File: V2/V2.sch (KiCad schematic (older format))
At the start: 183 parts, among them U1 Elite-C

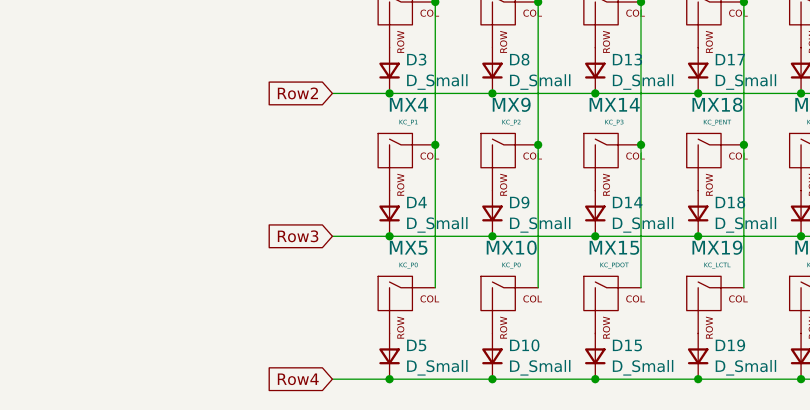
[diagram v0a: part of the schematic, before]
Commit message: Updated schematic and pcb design
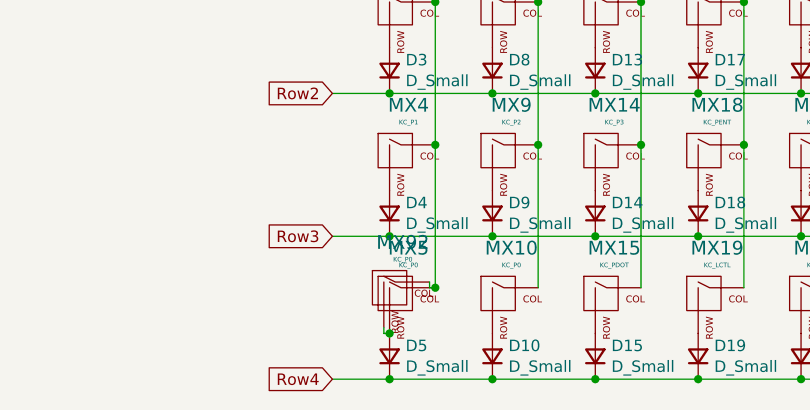
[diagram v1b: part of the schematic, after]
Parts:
- added MX92: KC_P0, MX_Alps_Hybrid:MXOnly-2U-Hotswap-ReversedStabilizers, symbol MX_Alps_Hybrid:MX-NoLED
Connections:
- net Col0: now also MX92.1 (COL)
- net at D5.2 (A), MX5.2 (ROW): now also MX92.2 (ROW)
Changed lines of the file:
@@
 Wire Wire Line
 	9075 2900 9975 2900
+$Comp
+L MX_Alps_Hybrid:MX-NoLED MX92
+U 1 1 60EC3BEF
+P 3275 3775
+F 0 "MX92" H 3308 3998 60  0000 C CNN
+F 1 "KC_P0" H 3308 3924 20  0000 C CNN
+F 2 "MX_Alps_Hybrid:MXOnly-2U-Hotswap-ReversedStabilizers" H 2650 3750 60  0001 C CNN
+F 3 "" H 2650 3750 60  0001 C CNN
+	1    3275 3775
+	1    0    0    -1
+$EndComp
+Wire Wire Line
+	3425 3725 3425 3750
+Wire Wire Line
+	3425 3750 3450 3750
+Connection ~ 3450 3750
+Wire Wire Line
+	3225 3925 3225 3950
+Wire Wire Line
+	3225 3950 3250 3950
+Connection ~ 3250 3950
 $EndSCHEMATC

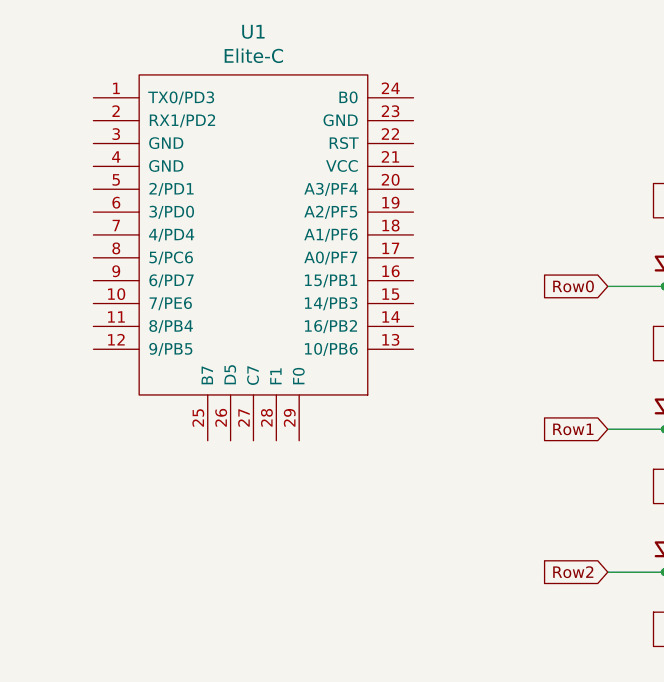
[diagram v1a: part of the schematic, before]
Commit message: Finished PCB
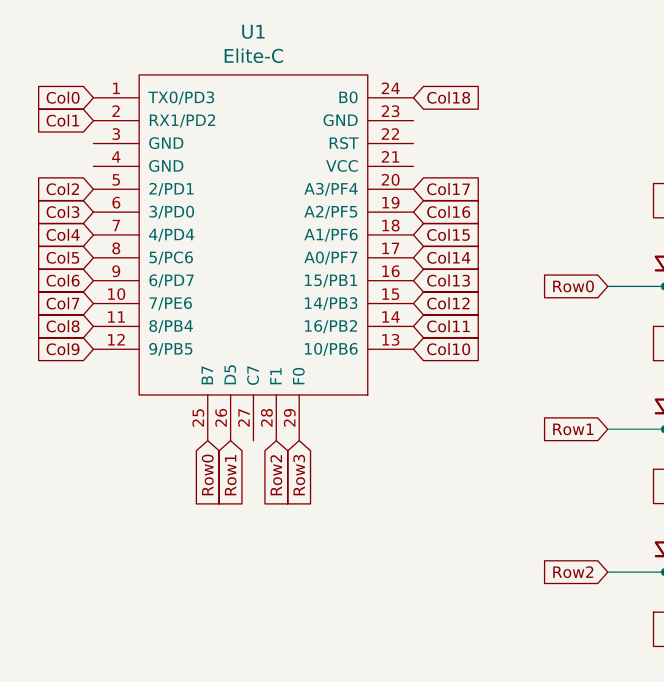
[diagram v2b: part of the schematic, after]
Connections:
- net Col0: now also U1.1 (TX0/PD3)
- net Col1: now also U1.2 (RX1/PD2)
- net Col10: now also U1.13 (10/PB6)
- net Col11: now also U1.14 (16/PB2)
- net Col12: now also U1.15 (14/PB3)
- net Col13: now also U1.16 (15/PB1)
- net Col14: now also U1.17 (A0/PF7)
- net Col15: now also U1.18 (A1/PF6)
- net Col16: now also U1.19 (A2/PF5)
- net Col17: now also U1.20 (A3/PF4)
- net Col18: now also U1.24 (B0)
- net Col2: now also U1.5 (2/PD1)
- net Col3: now also U1.6 (3/PD0)
- net Col4: now also U1.7 (4/PD4)
- net Col5: now also U1.8 (5/PC6)
- net Col6: now also U1.9 (6/PD7)
- net Col7: now also U1.10 (7/PE6)
- net Col8: now also U1.11 (8/PB4)
- net Col9: now also U1.12 (9/PB5)
- net Row0: now also U1.25 (B7)
- net Row1: now also U1.26 (D5)
- net Row2: now also U1.28 (F1)
- net Row3: now also U1.29 (F0)
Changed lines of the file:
@@
 	3225 3950 3250 3950
 Connection ~ 3250 3950
+Text GLabel 750  825  0    50   Input ~ 0
+Col0
+Text GLabel 750  925  0    50   Input ~ 0
+Col1
+Text GLabel 750  1225 0    50   Input ~ 0
+Col2
+Text GLabel 750  1325 0    50   Input ~ 0
+Col3
+Text GLabel 750  1425 0    50   Input ~ 0
+Col4
+Text GLabel 750  1525 0    50   Input ~ 0
+Col5
+Text GLabel 750  1725 0    50   Input ~ 0
+Col7
+Text GLabel 750  1825 0    50   Input ~ 0
+Col8
+Text GLabel 750  1925 0    50   Input ~ 0
+Col9
+Text GLabel 750  1625 0    50   Input ~ 0
+Col6
+Text GLabel 1250 2325 3    50   Input ~ 0
+Row0
+Text GLabel 1350 2325 3    50   Input ~ 0
+Row1
+Text GLabel 1550 2325 3    50   Input ~ 0
+Row2
+Text GLabel 1650 2325 3    50   Input ~ 0
+Row3
+Text GLabel 2150 825  2    50   Input ~ 0
+Col18
+Text GLabel 2150 1225 2    50   Input ~ 0
+Col17
+Text GLabel 2150 1325 2    50   Input ~ 0
+Col16
+Text GLabel 2150 1425 2    50   Input ~ 0
+Col15
+Text GLabel 2150 1525 2    50   Input ~ 0
+Col14
+Text GLabel 2150 1625 2    50   Input ~ 0
+Col13
+Text GLabel 2150 1725 2    50   Input ~ 0
+Col12
+Text GLabel 2150 1825 2    50   Input ~ 0
+Col11
+Text GLabel 2150 1925 2    50   Input ~ 0
+Col10
 $EndSCHEMATC

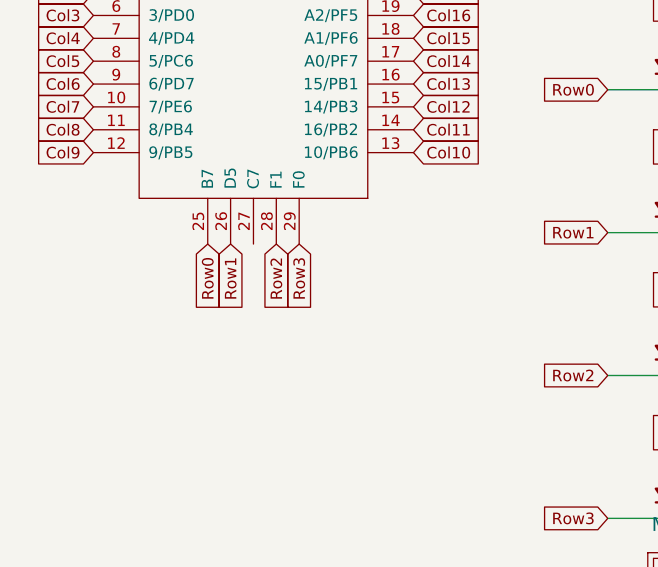
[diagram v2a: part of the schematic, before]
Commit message: Error Fixed
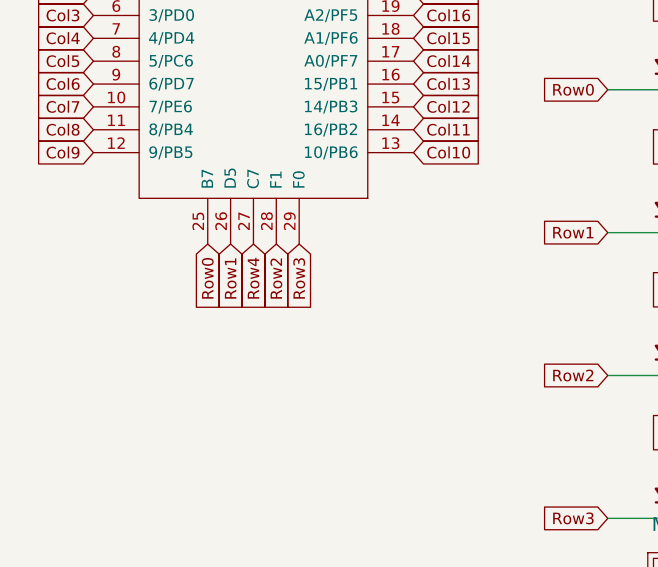
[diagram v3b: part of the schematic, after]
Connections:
- net Row4: now also U1.27 (C7)
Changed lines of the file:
@@
 Text GLabel 2150 1925 2    50   Input ~ 0
 Col10
+Text GLabel 1450 2325 3    50   Input ~ 0
+Row4
 $EndSCHEMATC
